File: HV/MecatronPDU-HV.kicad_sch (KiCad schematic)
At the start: 17 parts, among them J101 Power In, J102 PowerRelay, J103 SignalRelay, J104 Power Out, J105 Power Out, J106 Power Out, J107 Power Out, J108 Power Out, J109 Power Out

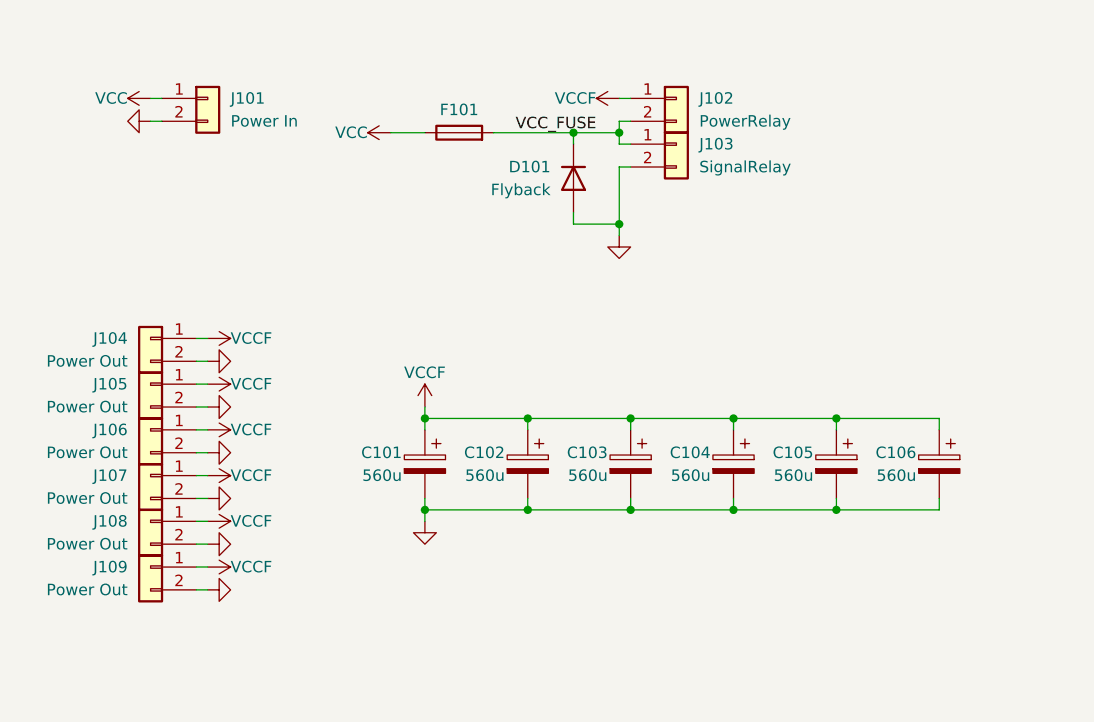
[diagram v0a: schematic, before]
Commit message: added HV
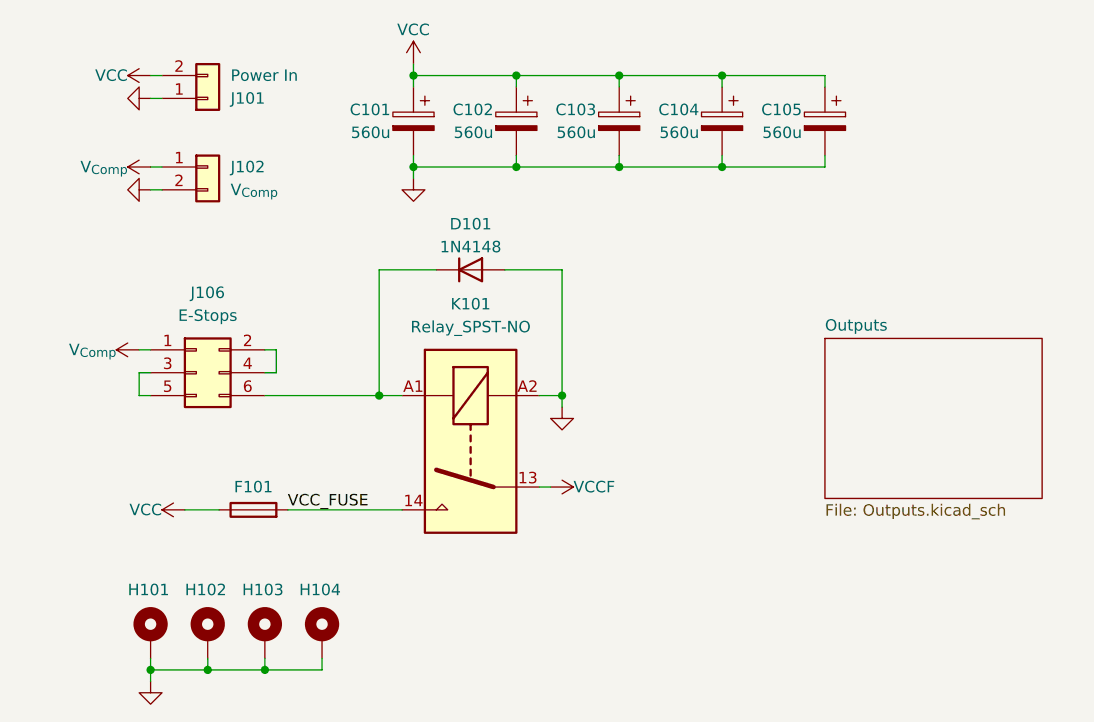
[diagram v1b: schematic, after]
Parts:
- removed C106: 560u, Capacitor_THT:CP_Radial_D10.0mm_P5.00mm, symbol Device:C_Polarized
- removed J103: SignalRelay, Connector_JST:JST_XH_B2B-XH-AM_1x02_P2.50mm_Vertical, symbol Connector_Generic:Conn_01x02
- removed J104, J105, J106, J107, J108, J109: Power Out, mecatron-kicad-footprints:AMASS_XT30PW-F_1x02_P2.50mm_Horizontal, symbol Connector_Generic:Conn_01x02
- added H101, H102, H103, H104: MountingHole_Pad_MP, MountingHole:MountingHole_5.3mm_M5_ISO7380_Pad_TopBottom, symbol Mechanical:MountingHole_Pad
- added J106: E-Stops, Connector_PinHeader_2.54mm:PinHeader_2x03_P2.54mm_Vertical, symbol Connector_Generic:Conn_02x03_Odd_Even
- added K101: Relay_SPST-NO, scottcjx-kicad-lib:G8PM1AW7RDC12, symbol Relay:Relay_SPST-NO
- C101, C102, C103, C104, C105: footprint Capacitor_THT:CP_Radial_D10.0mm_P5.00mm -> scottcjx-kicad-lib:CP_Radial_D10.0mm_P5.00mm
- D101: value Flyback -> 1N4148; footprint (none) -> Diode_THT:D_DO-35_SOD27_P7.62mm_Horizontal
- F101: footprint (none) -> scottcjx-kicad-lib:FUSE-MCCQ-122
- J101: footprint Connector_AMASS:AMASS_XT60PW-F_1x02_P7.20mm_Horizontal -> Connector_AMASS:AMASS_XT60-M_1x02_P7.20mm_Vertical
- J102: value PowerRelay -> V_{Comp}; footprint Connector_AMASS:AMASS_XT60PW-F_1x02_P7.20mm_Horizontal -> scottcjx-kicad-lib:JST_XH_B2B-XH-AM_1x02_P2.50mm_Vertical
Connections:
- net GND: now also J101.1 (Pin_1), J102.2 (Pin_2), H101.1, H102.1, H103.1, H104.1, K101.A2; no longer J101.2 (Pin_2)
- net VCC: now also C101.1, C102.1, C103.1, C104.1, C105.1, J101.2 (Pin_2); no longer J101.1 (Pin_1)
- net VCCF: now also K101.13; no longer C101.1, C102.1, C103.1, C104.1, C105.1, J102.1 (Pin_1)
- net VCC_FUSE: now also K101.14; no longer D101.1 (K), J102.2 (Pin_2)
- new net: D101.1 (K), J106.6 (Pin_6), K101.A1
- new net: J106.2 (Pin_2), J106.4 (Pin_4)
- new net: J106.3 (Pin_3), J106.5 (Pin_5)
- new net V_{Comp}: J102.1 (Pin_1), J106.1 (Pin_1)
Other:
- added sheet Outputs (Outputs.kicad_sch)
- company: (none) -> Scott CJX
- title: (none) -> Power Distribution Unit HV
